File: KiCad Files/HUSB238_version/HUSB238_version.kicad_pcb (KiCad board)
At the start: 2 copper layers, 54 x 12.9 mm, 33 parts, among them J2 2.54_PinHeader_02x02_SMD, J3 2.54_PinHeader_02x02_SMD, J4 2.5P Terminal Block, J9 USB_C_USB2.0_14P, Q2 AONR21307, Q9 AO3400A, SW1 SW_DIP_x05, U1 LM317L_SOT-89, U3 HUSB238_USB_PD, U4 USBLC6-2SC6

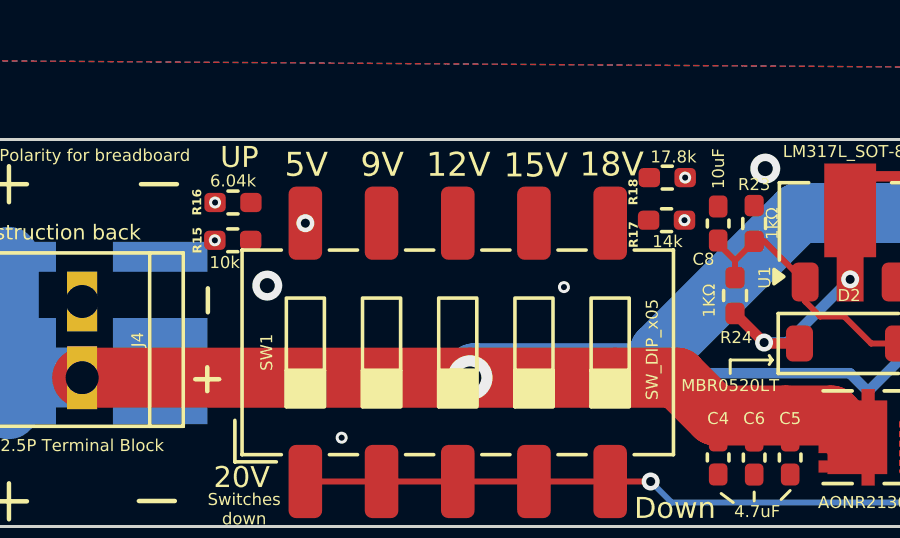
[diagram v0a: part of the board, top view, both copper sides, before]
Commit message: changed pcb
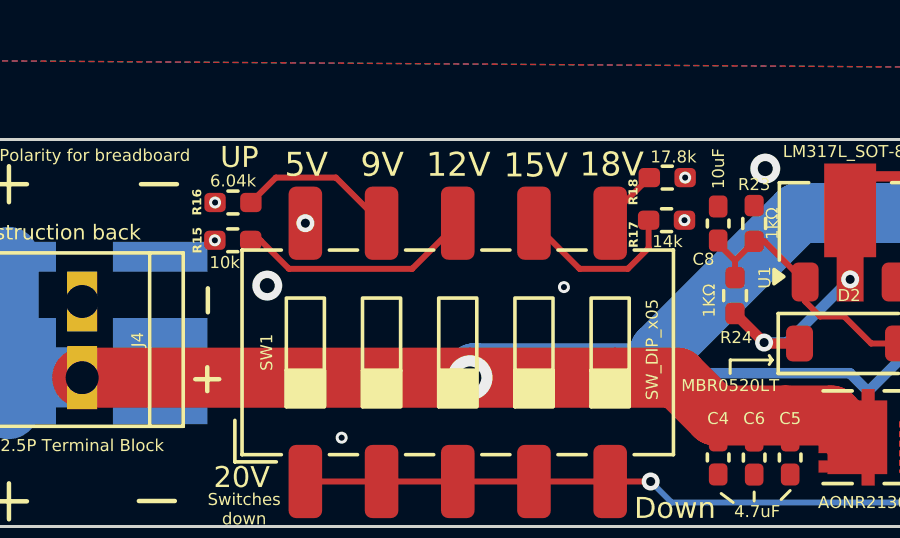
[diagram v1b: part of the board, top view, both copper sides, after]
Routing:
- net Net-(R15-Pad2): track 0.00 -> 7.93 mm
- net Net-(R17-Pad2): track 0.00 -> 5.67 mm
- net Net-(R16-Pad2): track 0.00 -> 5.33 mm
- net Net-(R18-Pad2): track 0.00 -> 2.06 mm
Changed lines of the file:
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@@
-		)
-	)
-	(dimension
-		(type orthogonal)
-		(layer "Dwgs.User")
-		(pts
-			(xy 193.07 116.87) (xy 140.37 116.58)
-		)
-		(height 6.67)
-		(orientation 0)
-		(format
-			(prefix "")
-			(suffix "")
-			(units 3)
-			(units_format 0)
-			(precision 4)
-			(suppress_zeroes yes)
-		)
-		(style
-			(thickness 0.1)
-			(arrow_length 1.27)
-			(text_position_mode 0)
-			(arrow_direction outward)
-			(extension_height 0.58642)
-			(extension_offset 0.5)
-			(keep_text_aligned yes)
-		)
-		(gr_text "52.7"
-			(at 166.72 122.39 0)
-			(layer "Dwgs.User")
-			(effects
-				(font
-					(size 1 1)
-					(thickness 0.15)
-				)
-			)
 		)
 	)
@@
 	)
 	(segment
+		(start 150.34384 110.76)
+		(end 151.29484 111.711)
+		(width 0.2)
+		(layer "F.Cu")
+		(net 13)
+	)
+	(segment
+		(start 155.399 111.711)
+		(end 156.92 110.19)
+		(width 0.2)
+		(layer "F.Cu")
+		(net 13)
+	)
+	(segment
+		(start 150.0175 110.76)
+		(end 150.34384 110.76)
+		(width 0.2)
+		(layer "F.Cu")
+		(net 13)
+	)
+	(segment
+		(start 151.29484 111.711)
+		(end 155.399 111.711)
+		(width 0.2)
+		(layer "F.Cu")
+		(net 13)
+	)
+	(segment
+		(start 150.856 108.669)
+		(end 150.025 109.5)
+		(width 0.2)
+		(layer "F.Cu")
+		(net 14)
+	)
+	(segment
+		(start 152.859 108.669)
+		(end 150.856 108.669)
+		(width 0.2)
+		(layer "F.Cu")
+		(net 14)
+	)
+	(segment
+		(start 154.38 110.19)
+		(end 152.859 108.669)
+		(width 0.2)
+		(layer "F.Cu")
+		(net 14)
+	)
+	(segment
+		(start 162.589 111.711)
+		(end 163.2825 111.0175)
+		(width 0.2)
+		(layer "F.Cu")
+		(net 15)
+	)
+	(segment
+		(start 160.981 111.711)
+		(end 162.589 111.711)
+		(width 0.2)
+		(layer "F.Cu")
+		(net 15)
+	)
+	(segment
+		(start 163.2825 111.0175)
+		(end 163.2825 110.09)
+		(width 0.2)
+		(layer "F.Cu")
+		(net 15)
+	)
+	(segment
+		(start 159.46 110.19)
+		(end 160.981 111.711)
+		(width 0.2)
+		(layer "F.Cu")
+		(net 15)
+	)
+	(segment
+		(start 162 110.19)
+		(end 162 109.975)
+		(width 0.2)
+		(layer "F.Cu")
+		(net 16)
+	)
+	(segment
+		(start 162 109.975)
+		(end 163.305 108.67)
+		(width 0.2)
+		(layer "F.Cu")
+		(net 16)
+	)
+	(segment
